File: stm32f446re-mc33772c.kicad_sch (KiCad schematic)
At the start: 50 parts, among them J1 Conn_01x02, J2 USB_B_Micro, J3 Conn_01x03, J4 Conn_01x03, J6 SM06B-GHS-TB, U1 STM32F446RET6, U3 LD1086D2M33TR, U4 AMS1117-3.3, U6 LMR51450SDRRR, U7 SN65HVD232, Y1 8MHz

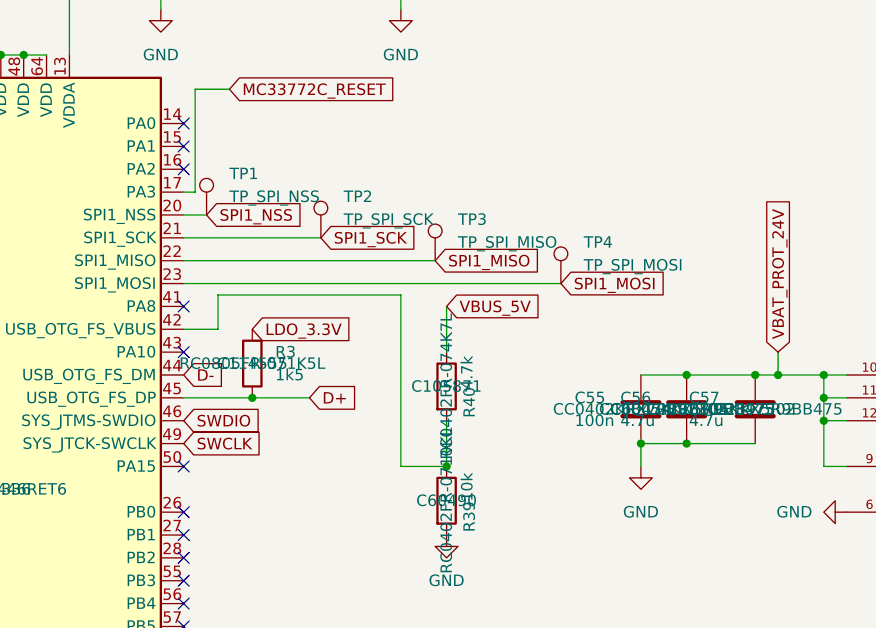
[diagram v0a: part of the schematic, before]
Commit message: cleanup sch
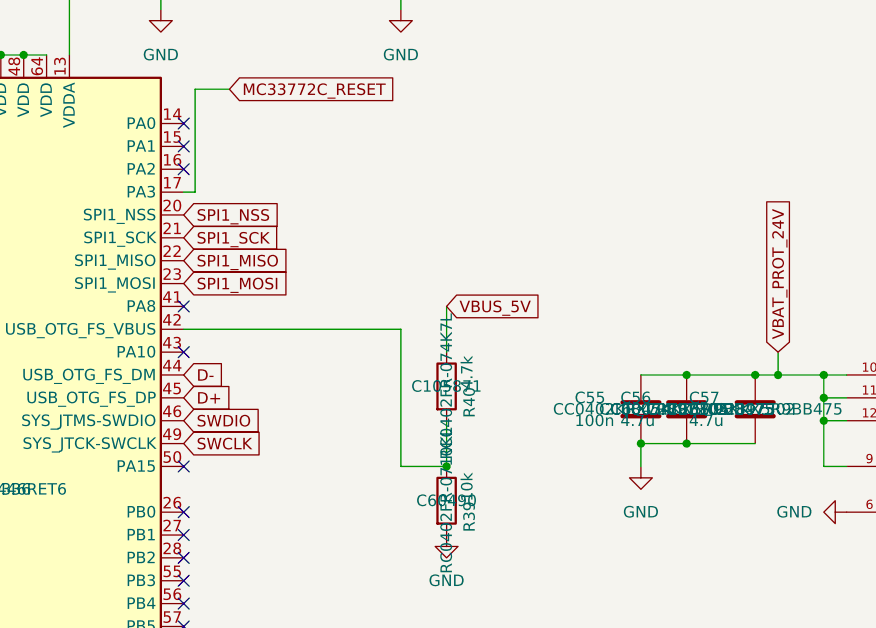
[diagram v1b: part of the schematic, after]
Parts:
- removed R3: 1k5, Resistor_SMD:R_0805_2012Metric, symbol Device:R
- removed TP1: TP_SPI_NSS, TestPoint:TestPoint_Pad_D1.0mm, symbol Connector:TestPoint
- removed TP2: TP_SPI_SCK, TestPoint:TestPoint_Pad_D1.0mm, symbol Connector:TestPoint
- removed TP3: TP_SPI_MISO, TestPoint:TestPoint_Pad_D1.0mm, symbol Connector:TestPoint
- removed TP4: TP_SPI_MOSI, TestPoint:TestPoint_Pad_D1.0mm, symbol Connector:TestPoint

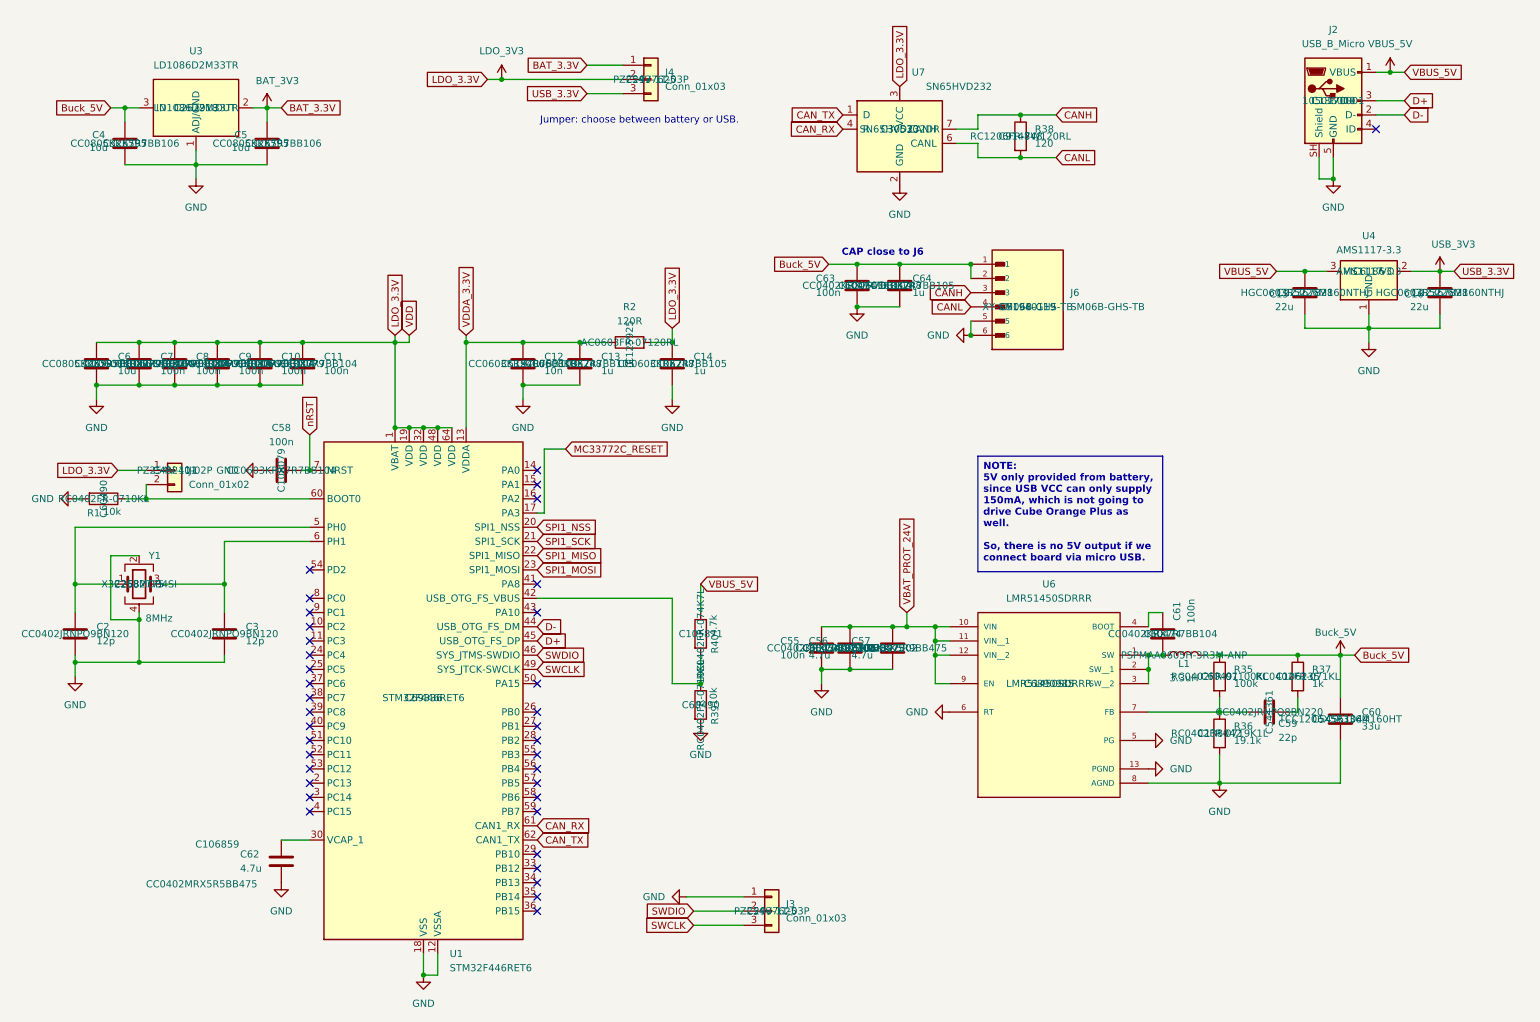
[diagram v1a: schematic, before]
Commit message: shrink, SWD
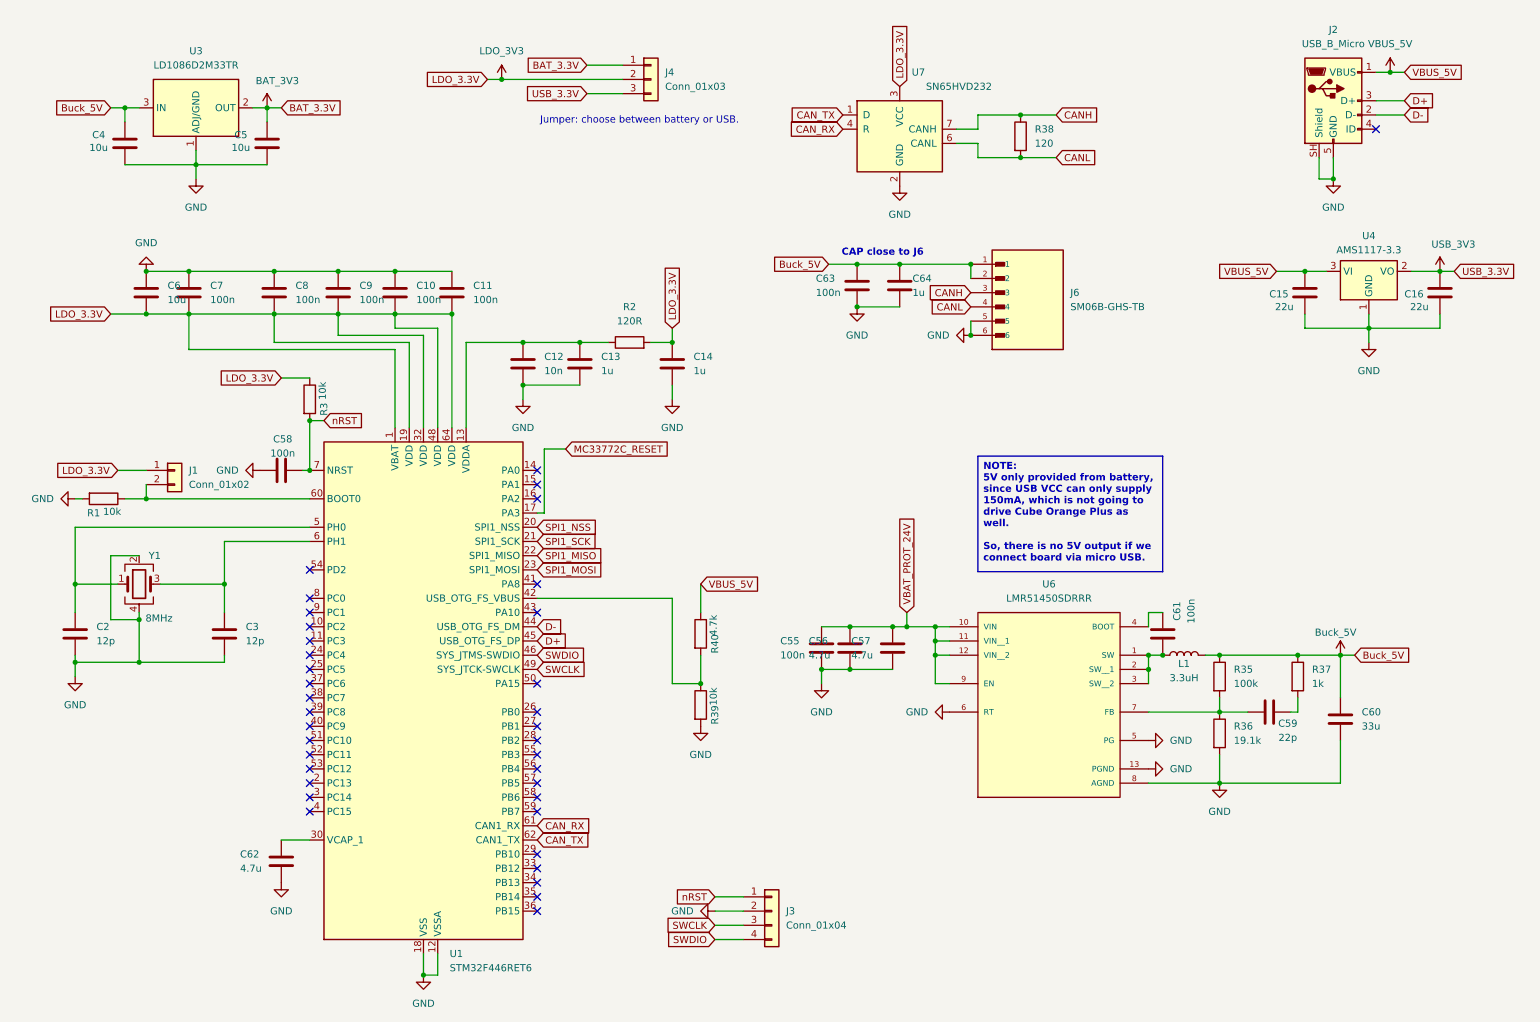
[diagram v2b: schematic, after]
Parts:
- added R3: 10k, Resistor_SMD:R_0402_1005Metric, symbol Device:R
- J3: value Conn_01x03 -> Conn_01x04; footprint Connector_PinHeader_2.54mm:PinHeader_1x03_P2.54mm_Vertical -> Connector_PinHeader_2.54mm:PinHeader_1x04_P2.54mm_Vertical; symbol Connector_Generic:Conn_01x03 -> Connector_Generic:Conn_01x04; FT Rotation Offset 90 -> (none); LCSC Part # C2937625 -> (none); MPN PZ254V-11-03P -> (none)
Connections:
- net GND: now also C10.1, C11.1, C6.1, C7.1, C8.1, C9.1, J3.2 (Pin_2); no longer C10.2, C11.2, C6.2, C7.2, C8.2, C9.2, J3.1 (Pin_1)
- net LDO_3V3: now also C10.2, C11.2, C6.2, C7.2, C8.2, C9.2, R3.1; no longer C10.1, C11.1, C6.1, C7.1, C8.1, C9.1
- net SWDIO: now also J3.4 (Pin_4); no longer J3.2 (Pin_2)
- net nRST: now also J3.1 (Pin_1), R3.2
- net VDDA_3.3V: no longer names the net of C12.1, C13.1, R2.1, U1.13 (VDDA)
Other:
- moved on the sheet: C6, C7
